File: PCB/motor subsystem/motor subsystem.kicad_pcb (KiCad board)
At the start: 2 copper layers, 100 x 100 mm, 33 parts, among them U1 MCU_Seeed_XIAO_ESP32-C3, U2 STP55NF06L

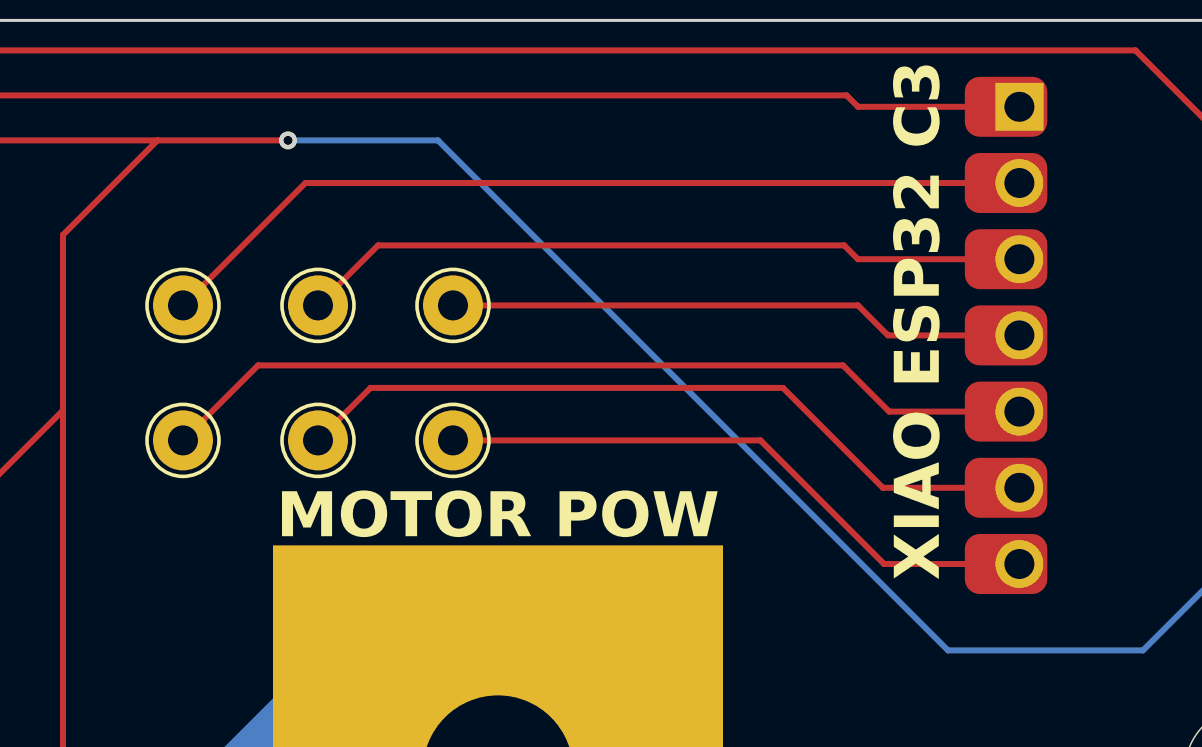
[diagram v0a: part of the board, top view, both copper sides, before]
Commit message: 07172025 - wrapping up CAD!
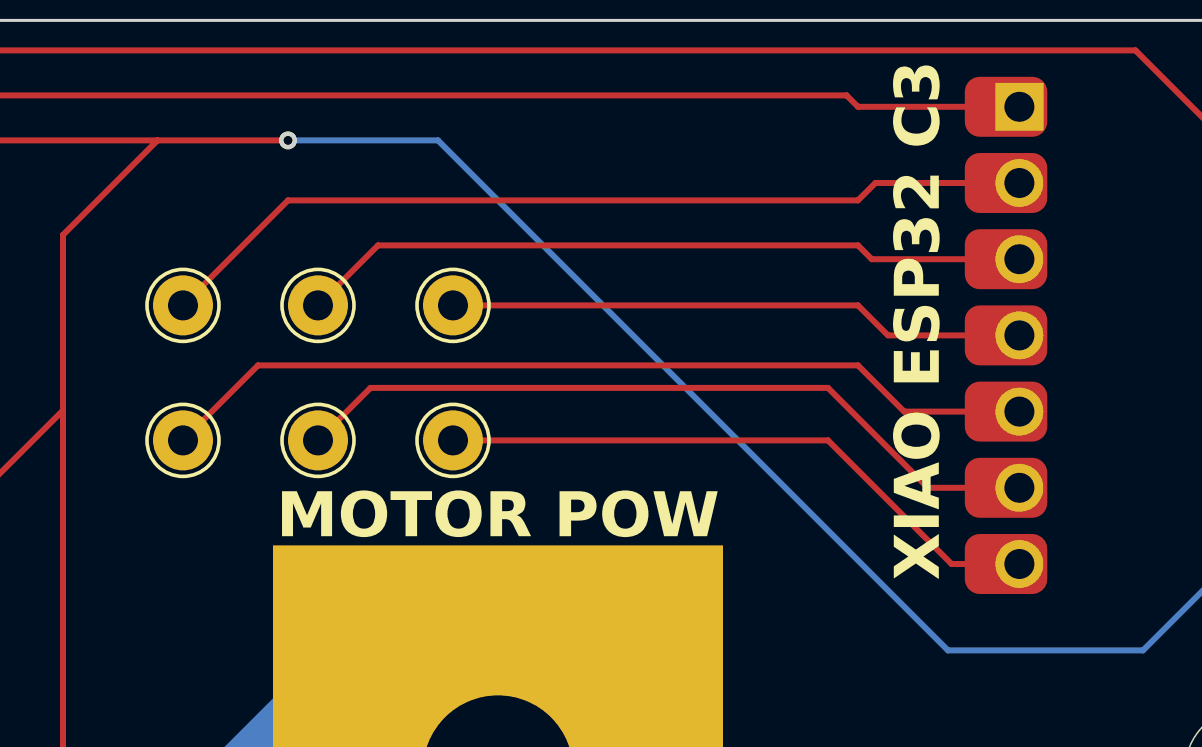
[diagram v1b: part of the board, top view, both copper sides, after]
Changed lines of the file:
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@@
 	)
 	(segment
-		(start 136.5 61.5)
-		(end 138.04 63.04)
-		(width 0.2)
-		(layer "F.Cu")
-		(net 20)
-	)
-	(segment
-		(start 138.04 63.04)
-		(end 142.38 63.04)
-		(width 0.2)
-		(layer "F.Cu")
-		(net 20)
-	)
-	(segment
-		(start 117 61.5)
-		(end 136.5 61.5)
+		(start 137 61.5)
+		(end 138.54 63.04)
 		(width 0.2)
 		(layer "F.Cu")
@@
 	)
 	(segment
-		(start 137.83 65.58)
+		(start 138.54 63.04)
+		(end 142.38 63.04)
+		(width 0.2)
+		(layer "F.Cu")
+		(net 20)
+	)
+	(segment
+		(start 117 61.5)
+		(end 137 61.5)
+		(width 0.2)
+		(layer "F.Cu")
+		(net 20)
+	)
+	(segment
+		(start 139.33 65.58)
 		(end 142.38 65.58)
 		(width 0.2)
@@
 	(segment
 		(start 120.75 62.25)
-		(end 134.5 62.25)
+		(end 136 62.25)
 		(width 0.2)
 		(layer "F.Cu")
@@
 	)
 	(segment
-		(start 134.5 62.25)
-		(end 137.83 65.58)
+		(start 136 62.25)
+		(end 139.33 65.58)
 		(width 0.2)
 		(layer "F.Cu")
@@
 	)
 	(segment
-		(start 137.87 68.12)
+		(start 140.12 68.12)
 		(end 142.38 68.12)
 		(width 0.2)
@@
 	)
 	(segment
-		(start 133.75 64)
-		(end 137.87 68.12)
+		(start 123.5 64)
+		(end 136 64)
 		(width 0.2)
 		(layer "F.Cu")
@@
 	)
 	(segment
-		(start 123.5 64)
-		(end 133.75 64)
+		(start 136 64)
+		(end 140.12 68.12)
 		(width 0.2)
 		(layer "F.Cu")
@@
 	)
 	(segment
-		(start 119 59.5)
-		(end 121 57.5)
+		(start 121 57.5)
+		(end 137 57.5)
 		(width 0.2)
 		(layer "F.Cu")
@@
 	)
 	(segment
-		(start 137 57.96)
+		(start 137 57.5)
+		(end 137.46 57.96)
+		(width 0.2)
+		(layer "F.Cu")
+		(net 23)
+	)
+	(segment
+		(start 137.46 57.96)
 		(end 142.38 57.96)
 		(width 0.2)
@@
 	)
 	(segment
-		(start 121 57.5)
-		(end 136.54 57.5)
-		(width 0.2)
-		(layer "F.Cu")
-		(net 23)
-	)
-	(segment
-		(start 136.54 57.5)
-		(end 137 57.96)
+		(start 119 59.5)
+		(end 121 57.5)
 		(width 0.2)
 		(layer "F.Cu")
@@
 	)
 	(segment
-		(start 114.5 59.5)
-		(end 118.58 55.42)
+		(start 137 56)
+		(end 137.58 55.42)
 		(width 0.2)
 		(layer "F.Cu")
@@
 	)
 	(segment
-		(start 118.58 55.42)
+		(start 137.58 55.42)
 		(end 142.38 55.42)
 		(width 0.2)
 		(layer "F.Cu")
+		(net 25)
+	)
+	(segment
+		(start 114.5 59.5)
+		(end 118 56)
+		(width 0.2)
+		(layer "F.Cu")
+		(net 25)
+	)
+	(segment
+		(start 118 56)
+		(end 137 56)
+		(width 0.2)
+		(layer "F.Cu")
